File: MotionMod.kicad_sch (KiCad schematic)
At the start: 20 parts, among them J1 HC-SR04 Ultrasonic, J2 Photoelectric Module, J3 MCP4728 12 Bit DAC, J4 CV Out 1, J5 CV Out 2, J6 CV Out 3, J7 CV Out 4, J8 AMS1117 3.3v Regulator, J9 Eurorack Power, U1 TL074

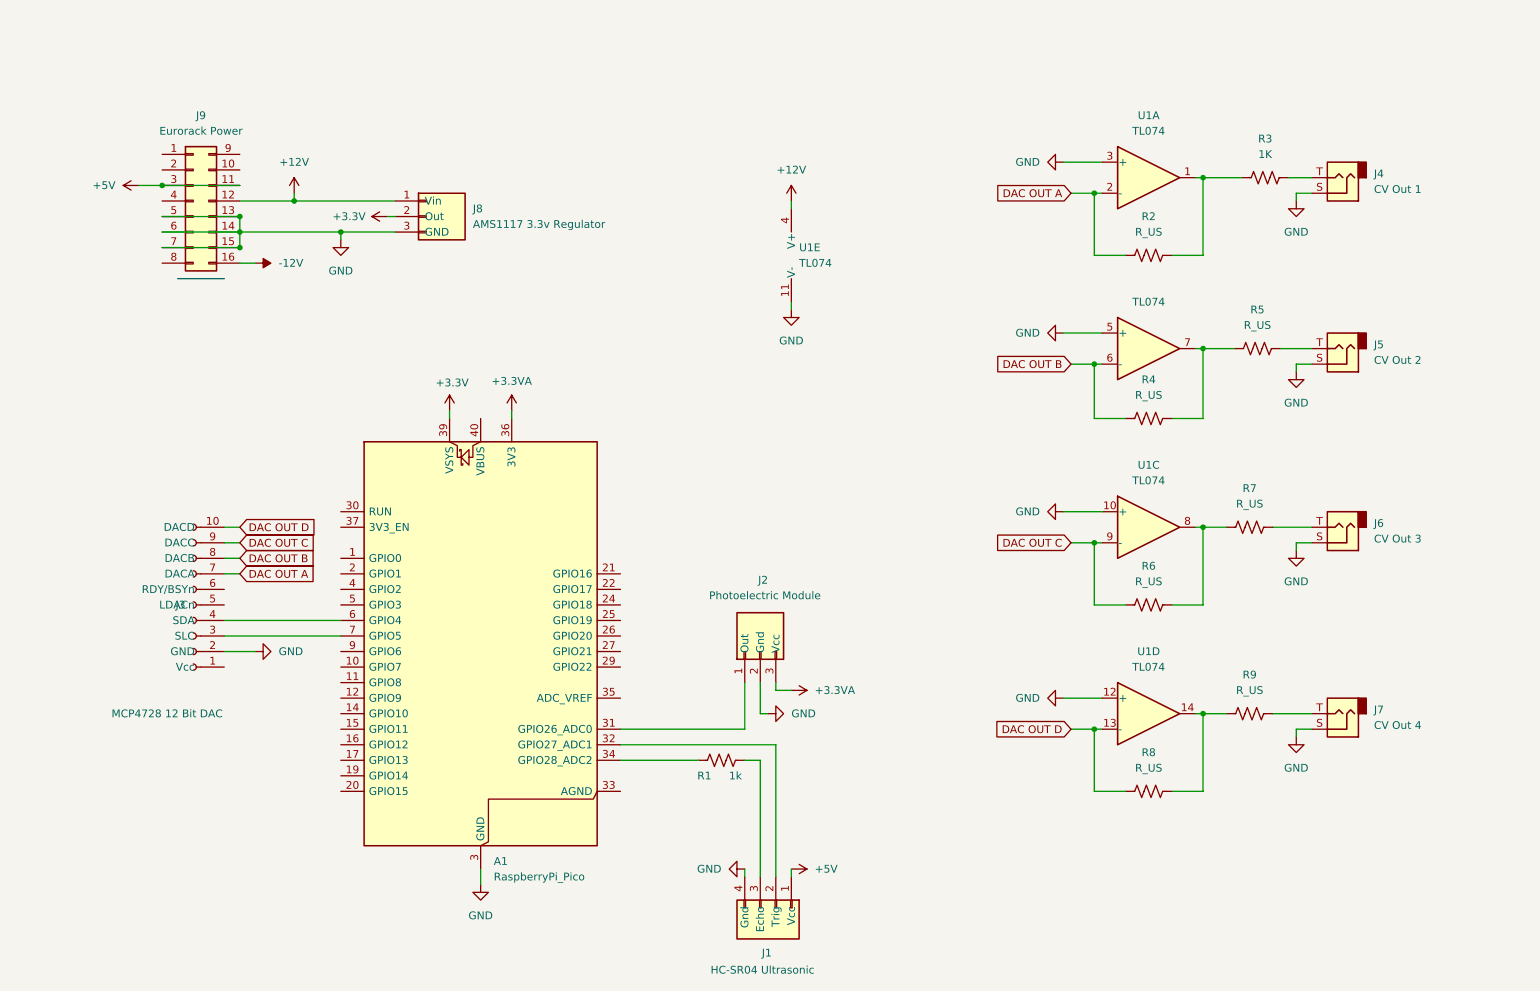
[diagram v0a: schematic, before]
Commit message: final gerbers for v1
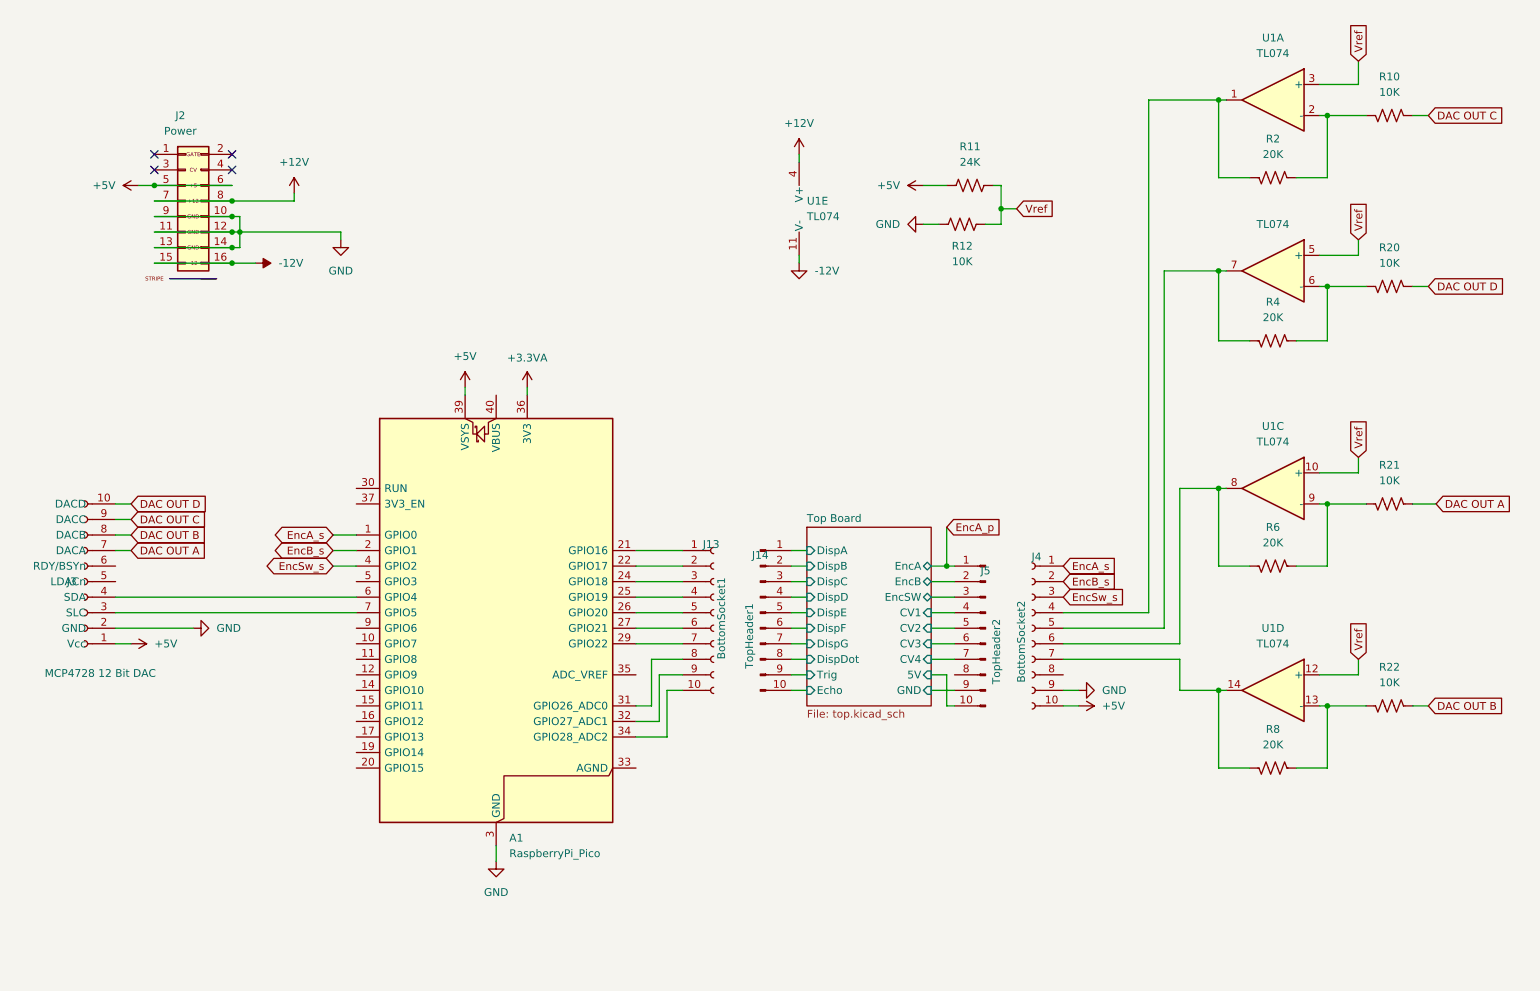
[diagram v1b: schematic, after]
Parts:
- removed J1: HC-SR04 Ultrasonic, symbol Connector_Generic:Conn_01x04
- removed J2: Photoelectric Module, symbol Connector_Generic:Conn_01x03
- removed J4: CV Out 1, symbol Connector_Audio:AudioJack2
- removed J5: CV Out 2, symbol Connector_Audio:AudioJack2
- removed J6: CV Out 3, symbol Connector_Audio:AudioJack2
- removed J7: CV Out 4, symbol Connector_Audio:AudioJack2
- removed J8: AMS1117 3.3v Regulator, symbol Connector_Generic:Conn_01x03
- removed R1: 1k, symbol Device:R_US
- removed R3: 1K, symbol Device:R_US
- removed R5, R7, R9: R_US, symbol Device:R_US
- added J13: BottomSocket1, Connector_PinSocket_2.54mm:PinSocket_1x10_P2.54mm_Vertical, symbol Connector:Conn_01x10_Socket
- added J14: TopHeader1, Connector_PinHeader_2.54mm:PinHeader_1x10_P2.54mm_Vertical, symbol Connector:Conn_01x10_Pin
- added J4: BottomSocket2, Connector_PinSocket_2.54mm:PinSocket_1x10_P2.54mm_Vertical, symbol Connector:Conn_01x10_Socket
- added J5: TopHeader2, Connector_PinHeader_2.54mm:PinHeader_1x10_P2.54mm_Vertical, symbol Connector:Conn_01x10_Pin
- added R10, R12, R20, R21, R22: 10K, PCM_4ms_Resistor:R_Axial_DIN0207_L6.3mm_D2.5mm_P7.62mm_Horizontal, symbol Device:R_US
- added R11: 24K, PCM_4ms_Resistor:R_Axial_DIN0207_L6.3mm_D2.5mm_P7.62mm_Horizontal, symbol Device:R_US
- A1: footprint Module:RaspberryPi_Pico_Common_Unspecified -> Module:RaspberryPi_Pico_SMD_HandSolder
- J2: renamed from J9; value Eurorack Power -> Power; footprint (none) -> PCM_4ms_Connector:Pins_2x08_2.54mm_TH_EuroPower; symbol Connector_Generic:Conn_02x08_Top_Bottom -> PCM_4ms_Connector:Eurorack_Power_16pin_Unshrouded; Manufacturer (none) -> TAD; Part Number (none) -> 1-1602FBV0T; Specifications (none) -> Header, Male Pins, 2*8, spacing 2.54mm, straight pin
- J3: footprint (none) -> Connector_PinHeader_2.54mm:PinHeader_1x10_P2.54mm_Vertical
- R2, R4, R6, R8: value R_US -> 20K; footprint (none) -> PCM_4ms_Resistor:R_Axial_DIN0207_L6.3mm_D2.5mm_P7.62mm_Horizontal
- U1: footprint (none) -> Package_DIP:DIP-14_W7.62mm_LongPads
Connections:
- net +3.3V is gone; now on net +5V: A1.39 (VSYS)
- net +12V: now also J2.7 (12V), J2.8 (+12V); no longer J2.12 (Pin_12)
- net +5V: now also J2.5 (+12V), J2.6 (P6), J3.1 (Vcc), J4.10 (Pin_10), R11.1; no longer J2.11 (Pin_11), J2.3 (Pin_3)
- net -12V: now also J2.15 (-12V), U1.11 (V-)
- net DAC OUT A: now also R21.1; no longer R2.1, U1.2 (-)
- net DAC OUT B: now also R22.1; no longer R4.1, U1.6 (-)
- net DAC OUT C: now also R10.1; no longer R6.1, U1.9 (-)
- net DAC OUT D: now also R20.1; no longer R8.1, U1.13 (-)
- net GND: now also J2.10 (GND), J2.11 (GND), J2.12 (GND), J2.9 (GND), J4.9 (Pin_9), R12.1; no longer J2.15 (Pin_15), J2.5 (Pin_5), J2.6 (Pin_6), J2.7 (Pin_7), U1.10 (+), U1.11 (V-), U1.12 (+), U1.3 (+), U1.5 (+)
- net EncA_s: now reaches A1.1 (GPIO0)
- net EncA_s: now also J4.1 (Pin_1)
- net EncB_s: now reaches A1.2 (GPIO1)
- net EncB_s: now also J4.2 (Pin_2)
- net at A1.21 (GPIO16): now also J13.1 (Pin_1)
- net at A1.22 (GPIO17): now also J13.2 (Pin_2)
- net at A1.24 (GPIO18): now also J13.3 (Pin_3)
- net at A1.25 (GPIO19): now also J13.4 (Pin_4)
- net at A1.26 (GPIO20): now also J13.5 (Pin_5)
- net at A1.27 (GPIO21): now also J13.6 (Pin_6)
- net at A1.29 (GPIO22): now also J13.7 (Pin_7)
- net at A1.31 (GPIO26_ADC0): now also J13.8 (Pin_8)
- net at A1.32 (GPIO27_ADC1): now also J13.9 (Pin_9)
- net at A1.34 (GPIO28_ADC2): now also J13.10 (Pin_10)
- net EncSw_s: now reaches A1.4 (GPIO2)
- net EncSw_s: now also J4.3 (Pin_3)
- net at R2.2, U1.1: now also J4.4 (Pin_4)
- net at R6.2, U1.8: now also J4.6 (Pin_6)
- net at R4.2, U1.7: now also J4.5 (Pin_5)
- net at R8.2, U1.14: now also J4.7 (Pin_7)
- new net: R21.2, R6.1, U1.9 (-)
- new net: R22.2, R8.1, U1.13 (-)
- new net: R10.2, R2.1, U1.2 (-)
- new net: R20.2, R4.1, U1.6 (-)
- new net EncA_p: J5.1 (Pin_1)
- new net Top Board/5V: J5.10 (Pin_10)
- new net Top Board/CV1: J5.4 (Pin_4)
- new net Top Board/CV2: J5.5 (Pin_5)
- new net Top Board/CV3: J5.6 (Pin_6)
- new net Top Board/CV4: J5.7 (Pin_7)
- new net Top Board/DispA: J14.1 (Pin_1)
- new net Top Board/DispB: J14.2 (Pin_2)
- new net Top Board/DispC: J14.3 (Pin_3)
- new net Top Board/DispD: J14.4 (Pin_4)
- new net Top Board/DispDot: J14.8 (Pin_8)
- new net Top Board/DispE: J14.5 (Pin_5)
- new net Top Board/DispF: J14.6 (Pin_6)
- new net Top Board/DispG: J14.7 (Pin_7)
- new net Top Board/Echo: J14.10 (Pin_10)
- new net Top Board/EncB: J5.2 (Pin_2)
- new net Top Board/EncSW: J5.3 (Pin_3)
- new net Top Board/GND: J5.9 (Pin_9)
- new net Top Board/Trig: J14.9 (Pin_9)
- new net Vref: R11.2, R12.2, U1.10 (+), U1.12 (+), U1.3 (+), U1.5 (+)
- no-connect marks 0 -> 4
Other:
- added sheet Top Board (top.kicad_sch)
- moved on the sheet: A1, J3, R2, R4, R6, R8, U1A, U1C, U1D, U1E
